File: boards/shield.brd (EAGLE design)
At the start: 102.5 x 66 mm, 18 parts, among them IC1 LM75, Q1 IPP114N03L, U1 TLC5925IDWR

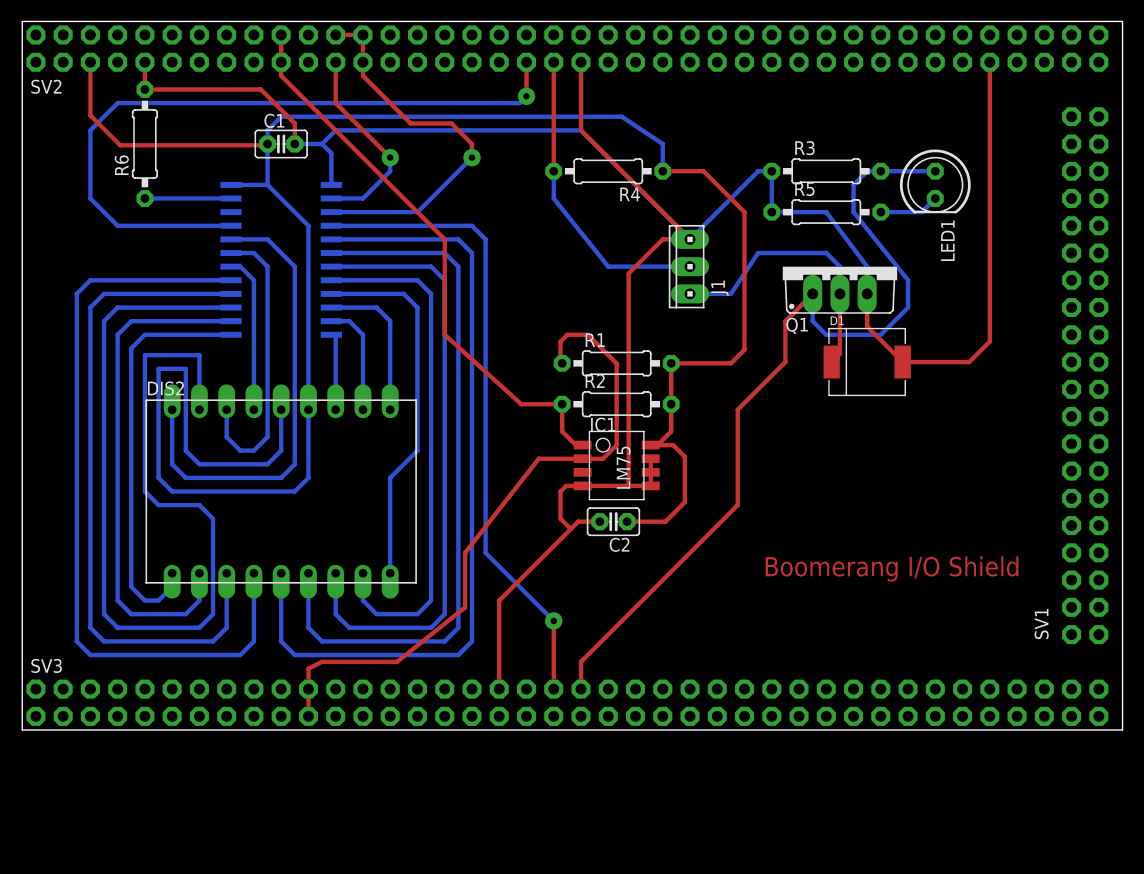
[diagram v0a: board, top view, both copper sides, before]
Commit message: put all the downloaded files into directories
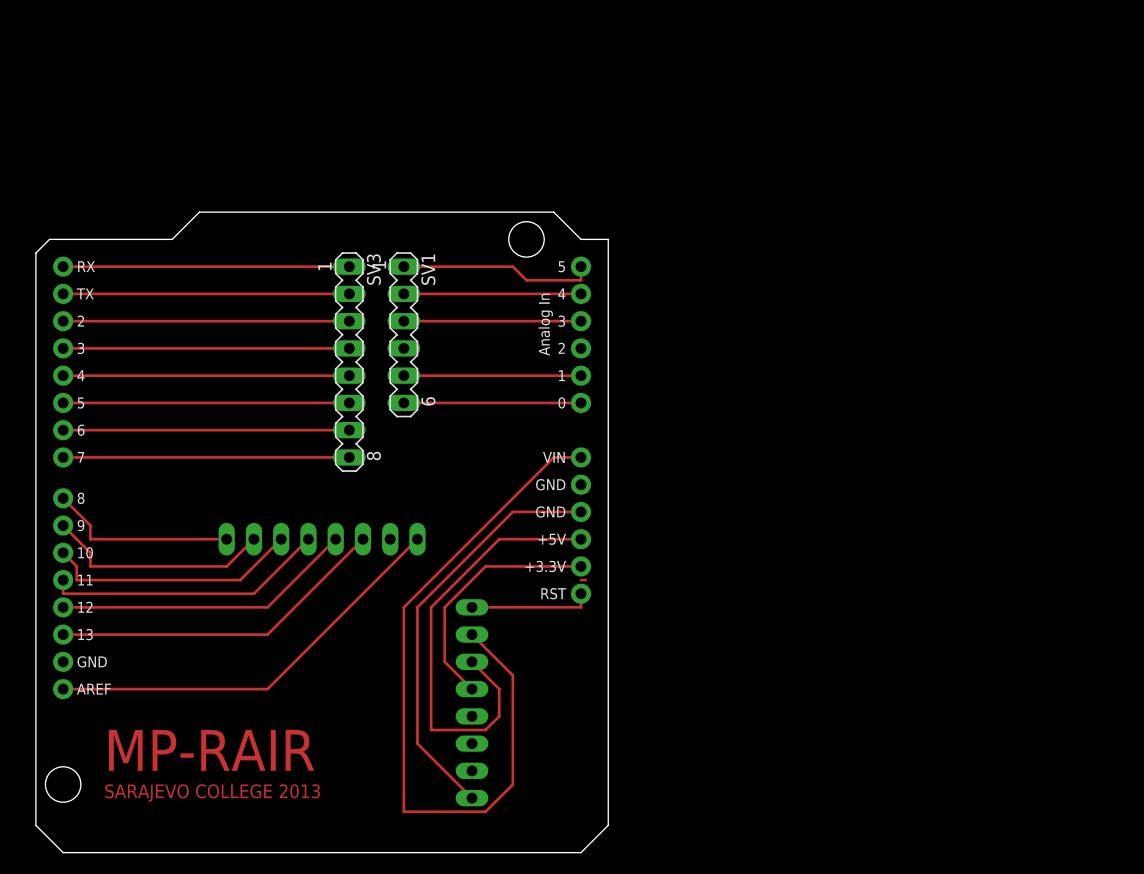
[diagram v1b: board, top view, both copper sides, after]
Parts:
- removed C1, C2: 100n, capacitor-wima:C2.5-2
- removed D1: 1.5SMCJ33A, seb:DO214AB
- removed DIS2: HDSP-521E, display-hp:HDSP-R
- removed IC1: LM75, lm75:SO8_LM75
- removed J1: (no value), con-amp:10X03MTA
- removed LED1: (no value), led:LED5MM
- removed Q1: IPP114N03L, transistor-power:TO220BV
- removed R1, R2, R3, R4: 10k, rcl:0207/10
- removed R5: 330, rcl:0207/10
- removed R6: 330R, rcl:0207/10
- added SV4: (no value), con-lstb:MA08-1
- SV1: device boomerang:MA20-2 -> con-lstb:MA06-1
- SV2, SV3: device boomerang:MA40-2 -> con-lstb:MA08-1
- U1: value TLC5925IDWR -> ARDUINO_SHIELDLABEL; device Texas Instruments_By_element14_Batch_1:SOIC127P1030X265-24N -> SparkFun-Boards:DUEMILANOVE_SHIELD
- moved SV1 63.6 mm to (34.3, 48.3), flipped to the top, turned to 270 degrees
- moved SV2 63.2 mm to (40.6, 14.0), turned to 90 degrees
- moved U1 59.8 mm to (0.00, 0.00), flipped to the top
- moved SV3 32.2 mm to (29.2, 45.7), flipped to the top, turned to 270 degrees
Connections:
- net P165 renamed N$3
- removed net +3V3: C1.1, C2.1, DIS2.13, DIS2.14, IC1.8, R1.2, R2.2, R4.1, SV2.6, U1.24
- removed net GND: C1.2, C2.2, D1.A, IC1.4, IC1.5, IC1.6, IC1.7, J1.1, Q1.S, R3.1, R5.1, R6.2, SV2.10, SV2.42, SV2.72, SV3.35, U1.1
- removed net N$14: DIS2.15, U1.18
- removed net N$3 (its old number): DIS2.7, U1.7
- removed net P100: SV2.49
- removed net P101: SV3.52
- removed net P103: SV3.51
- removed net P104: SV2.51
- removed net P105: SV3.54
- removed net P106: SV2.54
- removed net P107: SV3.53
- removed net P108: SV2.53
- removed net P109: SV3.56
- removed net P110: SV2.56
- removed net P112: SV2.55
- removed net P113: SV3.58
- removed net P114: SV2.58
- removed net P115: SV3.57
- removed net P117: SV3.60
- removed net P118: SV2.60
- removed net P119: SV3.59
- removed net P120: SV2.59
- removed net P121: SV3.62
- removed net P122: SV2.62
- removed net P123: SV3.61
- removed net P124: SV2.61
- removed net P125: SV3.64
- removed net P126: SV2.64
- removed net P127: SV3.63
- removed net P128: SV2.63
- removed net P13: SV3.8
- removed net P130: SV2.66
- removed net P131: SV3.65
- removed net P132: SV2.65
- removed net P133: SV3.68
- removed net P134: SV2.68
- removed net P135: SV3.67
- removed net P136: SV2.67
- removed net P137: SV3.70
- removed net P138: SV2.70
- removed net P139: SV3.69
- removed net P14: SV2.8
- removed net P140: SV2.69
- removed net P141: SV3.72
- removed net P143: SV3.71
- removed net P144: SV2.71
- removed net P145: SV3.74
- removed net P146: SV2.74
- removed net P148: SV2.73
- removed net P149: SV3.76
- removed net P15: SV3.7
- removed net P150: SV2.76
- removed net P151: SV3.75
- removed net P152: SV2.75
- removed net P153: SV3.78
- removed net P154: SV2.78
- removed net P155: SV3.77
- removed net P156: SV2.77
- removed net P157: SV3.80
- removed net P158: SV2.80
- removed net P159: SV3.79
- removed net P16: SV2.7
- removed net P161: SV1.2
- removed net P162: SV1.39
- removed net P163: SV1.1
- removed net P164: SV1.40
- removed net P166: SV1.37
- removed net P167: SV1.3
- removed net P168: SV1.38
- removed net P169: SV1.6
- removed net P17: SV3.10
- removed net P170: SV1.35
- removed net P172: SV1.36
- removed net P173: SV1.8
- removed net P174: SV1.33
- removed net P175: SV1.7
- removed net P176: SV1.34
- removed net P177: SV1.10
- removed net P178: SV1.31
- removed net P179: SV1.9
- removed net P180: SV1.32
- removed net P181: SV1.12
- removed net P182: SV1.29
- removed net P184: SV1.30
- removed net P185: SV1.14
- removed net P186: SV1.27
- removed net P187: SV1.13
- removed net P188: SV1.28
- removed net P189: SV1.16
- removed net P19: SV3.9
- removed net P190: SV1.25
- removed net P191: SV1.15
- removed net P192: SV1.26
- removed net P193: SV1.18
- removed net P194: SV1.23
- removed net P195: SV1.17
- removed net P196: SV1.24
- removed net P197: SV1.20
- removed net P198: SV1.21
- removed net P199: SV1.19
- removed net P20: SV2.9
- removed net P21: SV3.12
- removed net P22: SV2.12
- removed net P23: SV3.11
- removed net P24: SV2.11
- removed net P25: SV3.14
- removed net P27: SV3.13
- removed net P28: SV2.13
- removed net P29: SV3.16
- removed net P30: SV2.16
- removed net P31: SV3.15
- removed net P33: SV3.18
- removed net P34: SV2.18
- removed net P35: SV3.17
- removed net P36: SV2.17
- removed net P37: SV3.20
- removed net P38: SV2.20
- removed net P40: IC1.1, R2.1, SV2.19
- removed net P41: IC1.2, R1.1, SV3.22
- removed net P42: SV2.22
- removed net P43: SV3.21
- removed net P44: SV2.21
- removed net P45: SV3.24
- removed net P46: SV2.24, U1.2
- removed net P47: SV3.23
- removed net P48: SV2.23, U1.3
- removed net P49: SV3.26
- removed net P51: SV3.25
- removed net P52: SV2.25
- removed net P53: SV3.28
- removed net P54: SV2.28
- removed net P55: SV3.27
- removed net P56: SV2.27
- removed net P57: SV3.30
- removed net P59: SV3.29
- removed net P60: SV2.29
- removed net P61: SV3.32
- removed net P62: SV2.32
- removed net P63: SV3.31
- removed net P64: SV2.31
- removed net P65: SV3.34
- removed net P66: SV2.34
- removed net P67: SV3.33
- removed net P68: SV2.33
- removed net P69: SV3.36
- removed net P70: SV2.36
- removed net P72: SV2.35
- removed net P73: SV3.38
- removed net P74: SV2.38, U1.21
- removed net P75: SV3.37
- removed net P76: SV2.37
- removed net P77: SV3.40
- removed net P78: J1.2, R4.2, SV2.40
- removed net P79: SV3.39, U1.4
- removed net P8: SV2.3
- removed net P80: SV2.39
- removed net P81: SV3.42
- removed net P83: LED1.A, Q1.G, R3.2, SV3.41
- removed net P84: SV2.41
- removed net P85: SV3.44
- removed net P86: SV2.44
- removed net P87: SV3.43
- removed net P89: SV3.46
- removed net P90: SV2.46
- removed net P91: SV3.45
- removed net P92: SV2.45
- removed net P93: SV3.48
- removed net P95: SV3.47
- removed net P96: SV2.47
- removed net P97: SV3.50
- removed net P98: SV2.50
- removed net P99: SV3.49
- new net N$19: SV3.7, U1.D6
- new net N$21: SV4.1, U1.D8
- new net N$22: SV4.2, U1.D9
- new net N$23: SV4.3, U1.D10
- new net N$24: SV4.4, U1.D11
- new net N$25: SV4.5, U1.D12
- new net N$26: SV4.6, U1.D13
- new net N$28: SV4.8, U1.AREF
- net N$1: now also SV1.6, U1.A0; no longer DIS2.5, U1.5
- net N$10: now also SV2.5, U1.3.3V; no longer DIS2.2, U1.14
- net N$11: now also SV3.1, U1.RX; no longer DIS2.17, U1.15
- net N$12: now also SV3.2, U1.TX; no longer DIS2.3, U1.16
- net N$13: now also SV2.1, U1.GND@0; no longer DIS2.4, U1.17
- net N$15: now also SV3.3, U1.D2; no longer DIS2.16, U1.19
- net N$16: now also SV3.4, U1.D3; no longer DIS2.18, U1.20
- net N$17: now also SV3.5, U1.D4; no longer D1.K, J1.3, Q1.D
- net N$18: now also SV3.6, U1.D5; no longer LED1.K, R5.2
- net N$2: now also SV1.5, U1.A1; no longer DIS2.6, U1.6
- net N$20: now also SV3.8, U1.D7; no longer R6.1, U1.23
- net N$4: now also SV1.3, U1.A3; no longer DIS2.8, U1.8
- net N$5: now also SV1.2, U1.A4; no longer DIS2.9, U1.9
- net N$6: now also SV1.1, U1.A5; no longer DIS2.10, U1.10
- net N$7: now also SV2.8, U1.RES; no longer DIS2.11, U1.11
- net N$8: now also SV2.7, U1.VIN; no longer DIS2.12, U1.12
- net N$9: now also SV2.6, U1.5V; no longer DIS2.1, U1.13
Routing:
- net GND: track 219.4 -> 0.00 mm
- net +3V3: track 201.9 -> 0.00 mm
- net P83: track 80.1 -> 0.00 mm
- net P74: track 65.6 -> 0.00 mm
- net N$11: track 90.0 -> 26.7 mm
- net P41: track 61.3 -> 0.00 mm
- net N$8: track 7.39 -> 68.1 mm
- net P79: track 59.4 -> 0.00 mm, vias 1 -> 0
- net N$1: track 75.0 -> 16.5 mm
- net N$3 (its old number): track 57.2 -> 0.00 mm
- net P40: track 52.7 -> 0.00 mm
- net N$2: track 66.1 -> 16.5 mm
- net N$28: track 0.00 -> 38.8 mm
- net N$12: track 62.3 -> 26.7 mm
- net P48: track 35.6 -> 0.00 mm, vias 1 -> 0
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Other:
- board size 102.5 x 66 mm -> 53.3 x 59.7 mm
- board text added: "MP-RAIR"
- board text added: "SARAJEVO COLLEGE 2013"
- board text removed: "Boomerang I/O Shield"
